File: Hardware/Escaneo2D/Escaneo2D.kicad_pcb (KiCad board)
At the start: 2 copper layers, 50 x 51 mm, 11 parts, among them J1 OLED_I2C, J2 HC-SR04, J3 USB, J4 PWR, M1 Stepper_Motor_unipolar_5pin, U1 STM32-BlackPill, U2 ULN2003

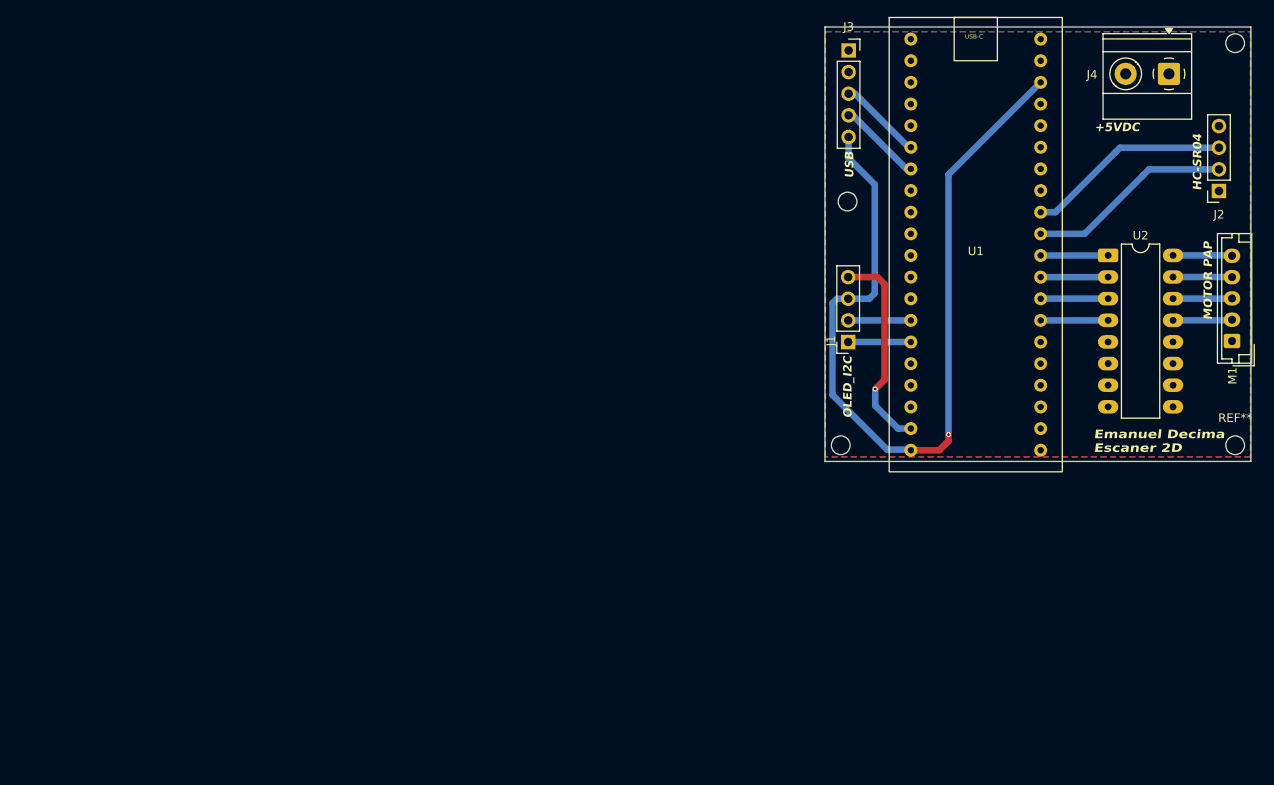
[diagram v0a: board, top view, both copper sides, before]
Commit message: PCB Terminada
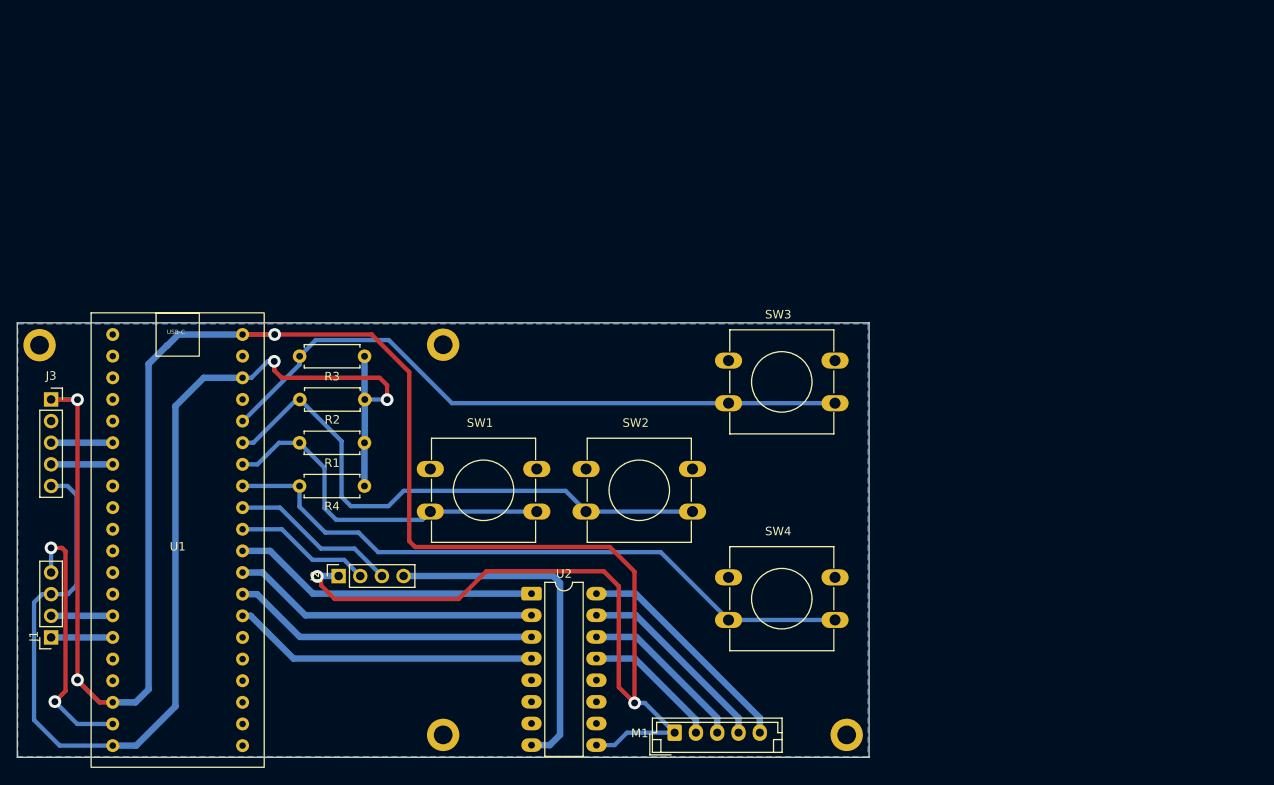
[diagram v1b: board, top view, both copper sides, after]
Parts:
- removed ? (x3): , 
- removed J4: PWR, TerminalBlock_Phoenix:TerminalBlock_Phoenix_MKDS-1,5-2-5.08_1x02_P5.08mm_Horizontal
- removed REF**: MountingHole_2.2mm_M2, MountingHole:MountingHole_2.2mm_M2
- added H1: MountingHole_Pad, MountingHole:MountingHole_2.2mm_M2_DIN965_Pad, F.Cu at (81.7, 124.3)
- added H2: MountingHole_Pad, MountingHole:MountingHole_2.2mm_M2_DIN965_Pad, F.Cu at (81.7, 170.2)
- added H3: MountingHole_Pad, MountingHole:MountingHole_2.2mm_M2_DIN965_Pad, F.Cu at (34.4, 124.4)
- added H4: MountingHole_Pad, MountingHole:MountingHole_2.2mm_M2_DIN965_Pad, F.Cu at (129.1, 170.2)
- added R1: 10K, Resistor_THT:R_Axial_DIN0207_L6.3mm_D2.5mm_P7.62mm_Horizontal, F.Cu at (72.5, 135.9)
- added R2: 10K, Resistor_THT:R_Axial_DIN0207_L6.3mm_D2.5mm_P7.62mm_Horizontal, F.Cu at (72.5, 130.8)
- added R3: 10K, Resistor_THT:R_Axial_DIN0207_L6.3mm_D2.5mm_P7.62mm_Horizontal, F.Cu at (72.5, 125.7)
- added R4: 10K, Resistor_THT:R_Axial_DIN0207_L6.3mm_D2.5mm_P7.62mm_Horizontal, F.Cu at (72.5, 140.9)
- added SW1: SW_Push, Button_Switch_THT:SW_PUSH-12mm, F.Cu at (80.2, 138.9)
- added SW2: SW_Push, Button_Switch_THT:SW_PUSH-12mm, F.Cu at (98.5, 138.9)
- added SW3: SW_Push, Button_Switch_THT:SW_PUSH-12mm, F.Cu at (115.2, 126.2)
- added SW4: SW_Push, Button_Switch_THT:SW_PUSH-12mm, F.Cu at (115.2, 151.7)
- moved J2 112.8 mm to (69.5, 151.5), turned to 90 degrees
- moved J3 102.2 mm to (35.7, 130.8)
- moved U1 99.9 mm to (50.6, 148.6)
- moved J1 99.8 mm to (35.7, 158.7)
- moved M1 80.0 mm to (108.9, 169.9), turned to 0 degrees
- moved U2 78.5 mm to (92.1, 153.6)
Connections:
- U1 pad 33: BTN_DOWN -> BTN_RETURN
- U1 pad 35: BTN_RETURN -> BTN_DOWN
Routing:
- net +5V: track 0.00 -> 265.4 mm, vias 0 -> 5
- net BTN_RETURN: track 0.00 -> 77.5 mm
- net BTN_ENTER: track 0.00 -> 77.1 mm
- net BTN_DOWN: track 0.00 -> 65.7 mm
- net GND: track 24.6 -> 71.2 mm, vias 1 -> 2
- net BTN_UP: track 0.00 -> 42.5 mm
- net +3V3: track 99.1 -> 137.1 mm, vias 1 -> 2
- net MOTOR_D: track 7.92 -> 36.0 mm
- net MOTOR_C: track 7.92 -> 36.0 mm
- net MOTOR_B: track 7.92 -> 36.0 mm
- net MOTOR_A: track 7.92 -> 36.0 mm
- net Net-(U2-O1): track 6.94 -> 27.0 mm
- net Net-(U2-O2): track 6.93 -> 23.4 mm
- net Net-(M1--): track 6.99 -> 19.9 mm
- net Net-(U2-O4): track 7.06 -> 16.2 mm
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- removed copper zone on F.Cu, net +5V
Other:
- board size 50 x 51 mm -> 100 x 51 mm
- board text removed: "+5VDC"
- board text removed: "Emanuel Decima Escaner 2D"
- board text removed: "HC-SR04"
- board text removed: "MOTOR PAP"
- board text removed: "OLED_I2C"
- board text removed: "USB"
